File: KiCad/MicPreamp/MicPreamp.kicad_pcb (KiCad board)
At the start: 2 copper layers, 23 x 19 mm, 19 parts, among them J1 PWR, J2 INT, J3 OUT, J4 AUX, J5 MIC, U1 MAX4062, U2 LT3042

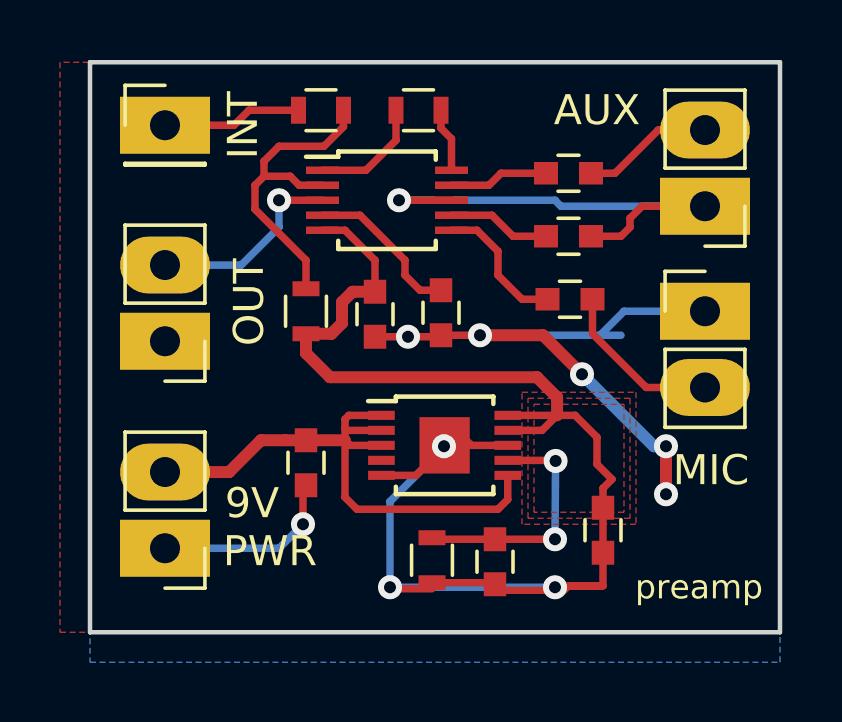
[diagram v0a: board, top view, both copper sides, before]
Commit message: Fix Preamp board
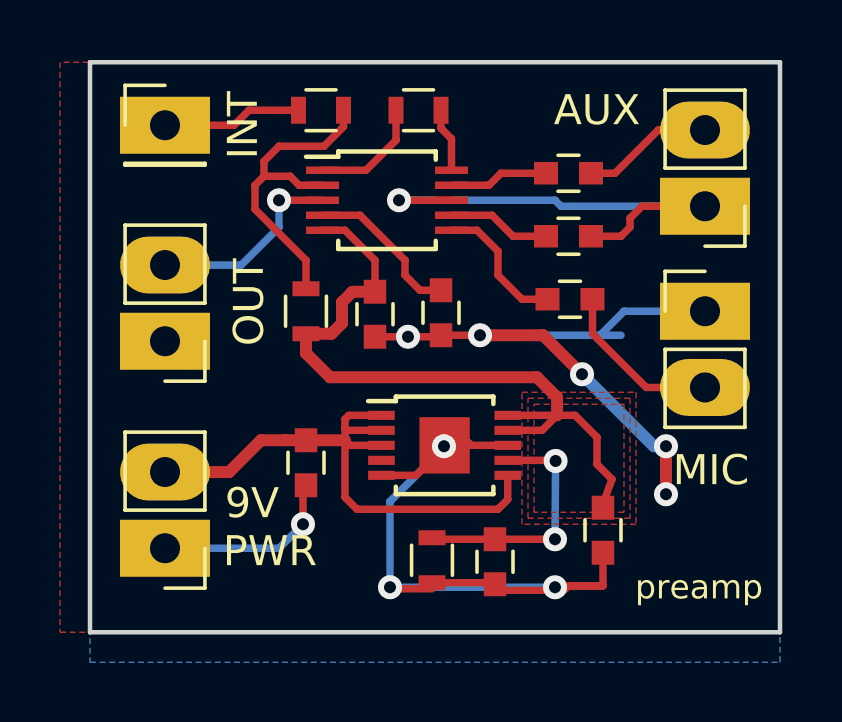
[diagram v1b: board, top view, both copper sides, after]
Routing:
- net VCC: track 25.6 -> 24.6 mm
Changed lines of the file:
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@@
     (thickness 1.6)
     (drawings 15)
-    (tracks 153)
+    (tracks 152)
     (zones 0)
     (modules 19)
@@
   (segment (start 143.07 73.27) (end 141.925 73.27) (width 0.25) (layer F.Cu) (net 10))
   (segment (start 143.57 72.77) (end 143.07 73.27) (width 0.25) (layer F.Cu) (net 10))
-  (segment (start 145.4 74.9) (end 144.9 74.4) (width 0.25) (layer F.Cu) (net 10))
-  (segment (start 144.9 74.4) (end 144.9 73.5) (width 0.25) (layer F.Cu) (net 10))
-  (segment (start 144.17 72.77) (end 143.57 72.77) (width 0.25) (layer F.Cu) (net 10))
-  (segment (start 144.9 73.5) (end 144.17 72.77) (width 0.25) (layer F.Cu) (net 10))
-  (segment (start 145.1 75.2) (end 145.4 74.9) (width 0.25) (layer F.Cu) (net 10))
-  (segment (start 145.1 76.95) (end 145.1 75.2) (width 0.25) (layer F.Cu) (net 10))
   (segment (start 135.2 70.05) (end 135.2 70.7) (width 0.4) (layer F.Cu) (net 10))
   (segment (start 135.2 70.7) (end 136 71.5) (width 0.4) (layer F.Cu) (net 10))
@@
   (segment (start 137.5 67.6) (end 137.5 68.65) (width 0.25) (layer F.Cu) (net 10))
   (segment (start 136.5 66.6) (end 137.5 67.6) (width 0.25) (layer F.Cu) (net 10))
+  (segment (start 144.17 72.77) (end 143.57 72.77) (width 0.25) (layer F.Cu) (net 10))
+  (segment (start 144.9 73.5) (end 144.17 72.77) (width 0.25) (layer F.Cu) (net 10))
+  (segment (start 144.9 74.4) (end 144.9 73.5) (width 0.25) (layer F.Cu) (net 10))
+  (segment (start 145 76) (end 145.4 74.9) (width 0.25) (layer F.Cu) (net 10))
+  (segment (start 145.4 74.9) (end 144.9 74.4) (width 0.25) (layer F.Cu) (net 10))
   (segment (start 134.75 62.6) (end 134.95 62.4) (width 0.25) (layer F.Cu) (net 11))
   (segment (start 133.3 62.6) (end 134.75 62.6) (width 0.25) (layer F.Cu) (net 11))
